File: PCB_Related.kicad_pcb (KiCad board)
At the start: 2 copper layers, 80 x 39 mm, 26 parts, among them SW1 SW_Push, U1 ATmega32U4RC-A, Y1 16MHz

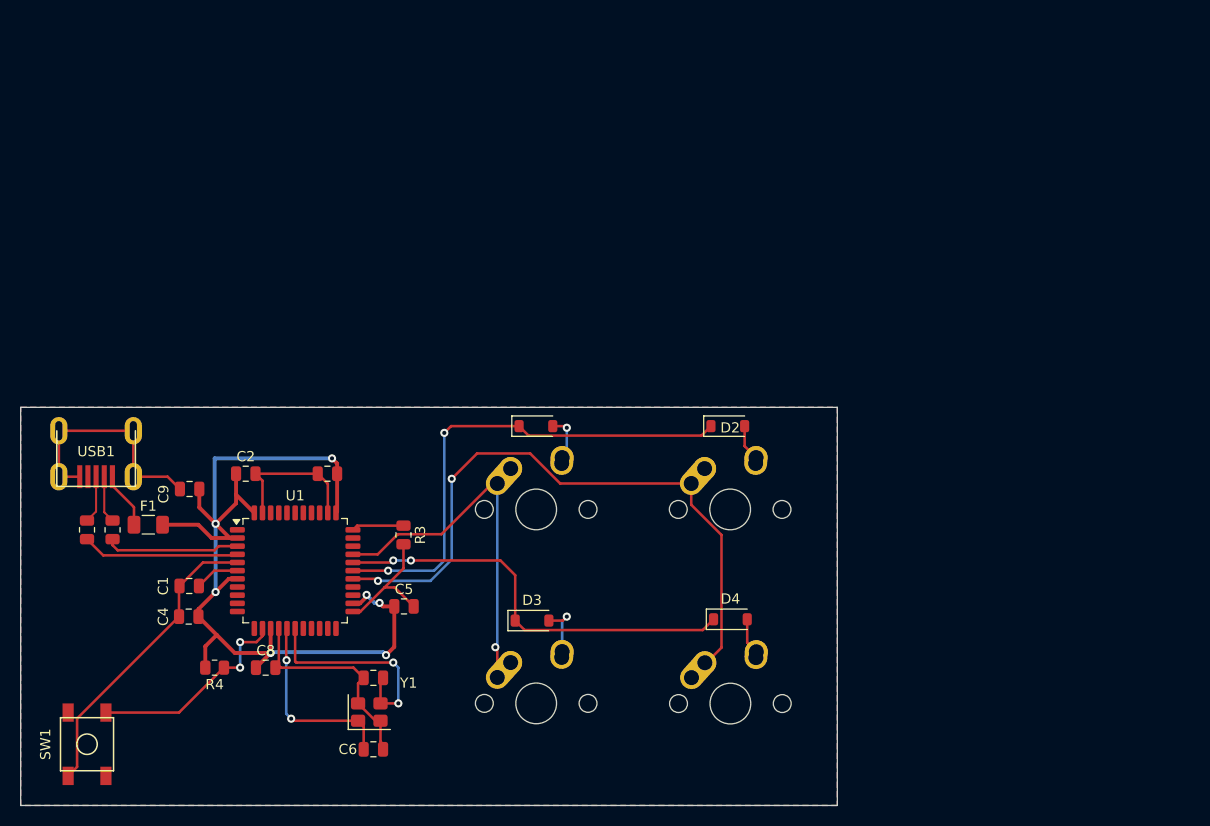
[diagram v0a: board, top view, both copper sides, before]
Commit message: Modified the PCB and added libraries
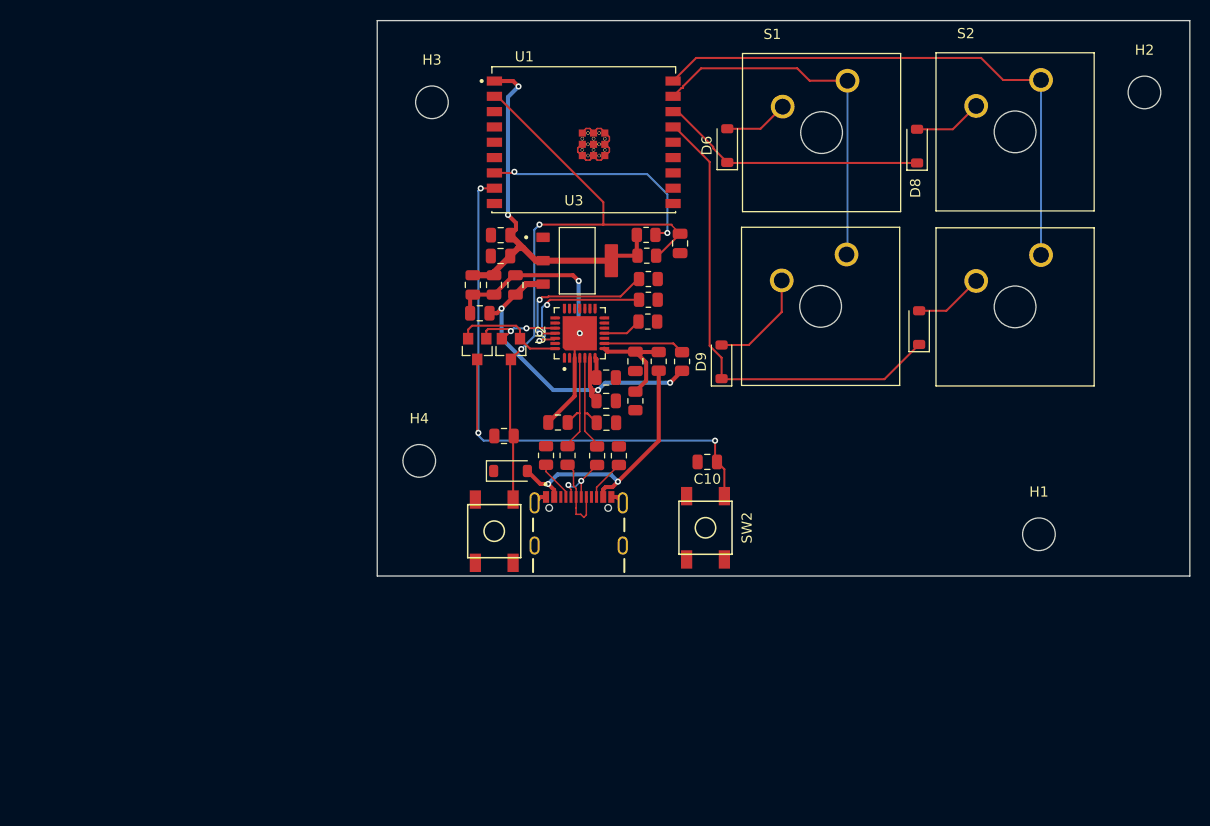
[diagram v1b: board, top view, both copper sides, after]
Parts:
- removed D1, D2, D4: SOD-123, Diode_SMD:D_SOD-123
- removed F1: 500mA, Fuse:Fuse_1206_3216Metric
- removed MX1, MX2, MX3, MX4: MX-NoLED, MX_Alps_Hybrid:MX-1U-NoLED
- removed R3, R4: 10K, Resistor_SMD:R_0805_2012Metric
- removed USB1: Molex-0548190589, random-keyboard-parts:Molex-0548190589
- removed Y1: 16MHz, Crystal:Crystal_SMD_3225-4Pin_3.2x2.5mm
- added C10: 0.1µF/50V, Capacitor_SMD:C_0805_2012Metric, F.Cu at (126.3, 64.8)
- added C11: 0.1µF/50V, Capacitor_SMD:C_0805_2012Metric, F.Cu at (107.5, 47.5)
- added C12: 10µF/25V, Capacitor_SMD:C_0805_2012Metric, F.Cu at (104.0, 50.3)
- added C13: 0.1µF/50V, Capacitor_SMD:C_0805_2012Metric, F.Cu at (105.4, 47.5)
- added C14: 10µF/25V, Capacitor_SMD:C_0805_2012Metric, F.Cu at (106.0, 44.7)
- added D10: Z1N5819HW-7-F, Diode_SMD:D_SOD-123, F.Cu at (147.0, 51.7)
- added D6: Z1N5819HW-7-F, Diode_SMD:D_SOD-123, F.Cu at (128.2, 33.9)
- added D8: Z1N5819HW-7-F, Diode_SMD:D_SOD-123, F.Cu at (146.8, 33.9)
- added D9: Z1N5819HW-7-F, Diode_SMD:D_SOD-123, F.Cu at (127.7, 55.0)
- added H1: MountingHole, MountingHole:MountingHole_3.2mm_M3, F.Cu at (158.8, 71.9)
- added H2: MountingHole, MountingHole:MountingHole_3.2mm_M3, F.Cu at (169.1, 28.7)
- added H3: MountingHole, MountingHole:MountingHole_3.2mm_M3, F.Cu at (99.3, 29.6)
- added H4: MountingHole, MountingHole:MountingHole_3.2mm_M3, F.Cu at (98.0, 64.7)
- added J1: USB4105-GF-A, USB4105-GF-A:GCT_USB4105-GF-A, F.Cu at (113.7, 73.0)
- added Q1: L8050QLT1G, SMD-TRANSISTORS-NPN-25V-500MW_SOT-23_:SOT-23, F.Cu at (107.0, 53.8)
- added Q2: L8050QLT1G, SMD-TRANSISTORS-NPN-25V-500MW_SOT-23_:SOT-23, F.Cu at (103.7, 53.8)
- added R10: 1K, Resistor_SMD:R_0805_2012Metric, F.Cu at (120.4, 51.1)
- added R11: 22.1K, Resistor_SMD:R_0805_2012Metric, F.Cu at (121.5, 55.0)
- added R12: 47.5K, Resistor_SMD:R_0805_2012Metric, F.Cu at (119.2, 58.9)
- added R13: 0, Resistor_SMD:R_0805_2012Metric, F.Cu at (120.5, 46.9)
- added R14: 0, Resistor_SMD:R_0805_2012Metric, F.Cu at (120.5, 49.0)
- added R15: 10K, Resistor_SMD:R_0805_2012Metric, F.Cu at (120.3, 44.6)
- added R16: 10K, Resistor_SMD:R_0805_2012Metric, F.Cu at (120.3, 42.6)
- added R7: 0, Resistor_SMD:R_0805_2012Metric, F.Cu at (112.6, 64.2)
- added R8: 0, Resistor_SMD:R_0805_2012Metric, F.Cu at (115.5, 64.2)
- added R9: 10K, Resistor_SMD:R_0805_2012Metric, F.Cu at (123.8, 55.0)
- added S1: MX1A-11NN, MX1A-11NN:SW_MX1A-11NN, F.Cu at (137.5, 32.6)
- added S2: MX1A-11NN, MX1A-11NN:SW_MX1A-11NN, F.Cu at (156.4, 32.5)
- added S3: MX1A-11NN, MX1A-11NN:SW_MX1A-11NN, F.Cu at (137.4, 49.6)
- added S4: MX1A-11NN, MX1A-11NN:SW_MX1A-11NN, F.Cu at (156.4, 49.7)
- added SW2: SW_Push, random-keyboard-parts:SKQG-1155865, F.Cu at (126.1, 71.3)
- added U2: CP2102N-A02-GQFN28R, CP2102N-A02-GQFN28R:IC_CP2102N-A02-GQFN28R, F.Cu at (113.8, 52.2)
- added U3: AMS1117-3.3, AMS1117-3.3:SOT229P700X180-4N, F.Cu at (113.5, 45.1)
- C1: value 1µF -> 22pF
- C2: value 0.1µF -> 22pF
- C3, C5: value 0.1µF -> 10µF/25V
- C4, C8: value 0.1µF -> 1µF/16V
- C6: value 22pF -> 0.1µF/50V
- C7: value 22pF -> 10µF/25V
- C9: value 0.1µF -> 0.1µF/50V
- D3: value SOD-123 -> LESD5D5.0CT1G
- R1, R2: value 22 -> 51k
- U1: value ATmega32U4RC-A -> ESP32-C3-WROOM-02U-N4; footprint Package_QFP:TQFP-44_10x10mm_P0.8mm -> ESP32-C3-WROOM-02U-N4:XCVR_ESP32-C3-WROOM-02U-N4
- moved C8 58.1 mm to (123.6, 43.4), turned to -90 degrees
- moved R1 52.6 mm to (117.6, 64.2), turned to 90 degrees
- moved U1 50.8 mm to (114.2, 33.3)
- moved C4 50.4 mm to (119.2, 55.0), turned to 90 degrees
- moved C6 46.5 mm to (103.3, 47.5), turned to -90 degrees
- moved C7 45.1 mm to (106.0, 42.6), turned to 180 degrees
- moved SW1 45.0 mm to (105.4, 71.6), turned to 90 degrees
- moved C1 43.9 mm to (116.4, 61.0), turned to 0 degrees
- moved R2 43.1 mm to (110.5, 64.2), turned to 90 degrees
- moved C9 31.2 mm to (106.3, 62.3)
- moved C2 31.0 mm to (111.6, 61.0), turned to 180 degrees
- moved C5 29.9 mm to (116.4, 56.6), turned to 180 degrees
- moved C3 28.2 mm to (116.4, 58.9), turned to 0 degrees
- moved D3 14.8 mm to (107.0, 65.7)
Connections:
- C1 pad 1: Net-(U1-UCAP) -> USB_DN
- C2 pad 1: +5V -> USB_DP
- C3 pad 1: +5V -> +3V3
- C4 pad 1: +5V -> GND
- C4 pad 2: GND -> Net-(U2-VBUS)
- C5 pad 1: +5V -> GND
- C5 pad 2: GND -> +3V3
- C6 pad 1: GND -> +3V3
- C6 pad 2: Net-(U1-XTAL2) -> GND
- C7 pad 1: GND -> +3V3
- C7 pad 2: Net-(U1-XTAL1) -> GND
- C8 pad 1: +5V -> CHIP_PU
- C9 pad 1: +5V -> CHIP_PU
- D3 pad 1: ROW1 -> GND
- D3 pad 2: Net-(D3-A) -> VBUS
- R1 pad 1: D+ -> Net-(J1-CC2)
- R1 pad 2: Net-(U1-D+) -> GND
- R2 pad 1: D- -> Net-(J1-CC1)
- R2 pad 2: Net-(U1-D-) -> GND
- SW1 pad 1: GND -> CHIP_PU
- SW1 pad 2: Net-(U1-~{RESET}) -> GND
- U1 pad 1: unconnected-(U1-PE6-Pad1) -> +3V3
- U1 pad 11: unconnected-(U1-PB3-Pad11) -> U0RXD
- U1 pad 12: unconnected-(U1-PB7-Pad12) -> U0TXD
- U1 pad 13: Net-(U1-~{RESET}) -> unconnected-(U1-IO18-Pad13)
- U1 pad 14: +5V -> unconnected-(U1-IO19-Pad14)
- U1 pad 15: GND -> ROW1
- U1 pad 16: Net-(U1-XTAL2) -> ROW0
- U1 pad 17: Net-(U1-XTAL1) -> COL0
- U1 pad 18: unconnected-(U1-PD0-Pad18) -> COL1
- U1 pad 2: +5V -> CHIP_PU
- U1 pad 3: Net-(U1-D-) -> unconnected-(U1-IO4-Pad3)
- U1 pad 4: Net-(U1-D+) -> unconnected-(U1-IO5-Pad4)
- U1 pad 5: GND -> unconnected-(U1-IO6-Pad5)
- U1 pad 6: Net-(U1-UCAP) -> unconnected-(U1-IO7-Pad6)
- U1 pad 7: +5V -> GPIO8
- U1 pad 8: unconnected-(U1-PB0-Pad8) -> GPIO9
- U1 pad 9: unconnected-(U1-PB1-Pad9) -> GND
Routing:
- net +5V: track 97.1 -> 0.00 mm, vias 7 -> 0
- net +3V3: track 0.00 -> 77.3 mm, vias 0 -> 5
- net CHIP_PU: track 0.00 -> 62.9 mm, vias 0 -> 2
- net GPIO9: track 0.00 -> 62.3 mm, vias 0 -> 3
- net GND: track 101.8 -> 45.3 mm, vias 0 -> 2
- net VBUS: track 0.00 -> 26.6 mm, vias 0 -> 2
- net ROW0: track 49.0 -> 26.1 mm, vias 2 -> 0
- net GPIO8: track 0.00 -> 22.9 mm, vias 0 -> 2
- net Net-(U1-XTAL1): track 21.4 -> 0.00 mm, vias 2 -> 0
- net Net-(U1-~{RESET}): track 20.6 -> 0.00 mm, vias 2 -> 0
- net Net-(U1-XTAL2): track 18.8 -> 0.00 mm, vias 2 -> 0
- net Net-(U2-RXD): track 0.00 -> 15.6 mm, vias 0 -> 2
- net Net-(U1-D+): track 15.4 -> 0.00 mm
- net Net-(U2-TXD): track 0.00 -> 15.3 mm, vias 0 -> 2
- net Net-(U1-D-): track 13.2 -> 0.00 mm
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- removed copper zone on B.Cu, net GND
- removed copper zone on F.Cu, net GND
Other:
- board size 80 x 39 mm -> 79.6 x 54.4 mm
- copper layers 2 -> 4
